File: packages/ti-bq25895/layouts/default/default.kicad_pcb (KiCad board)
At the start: 2 copper layers, 4 parts

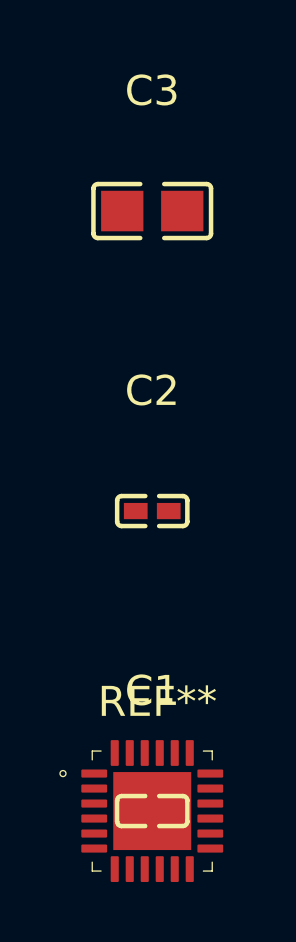
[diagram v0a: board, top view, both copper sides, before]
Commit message: adding has_part_picked trait to all
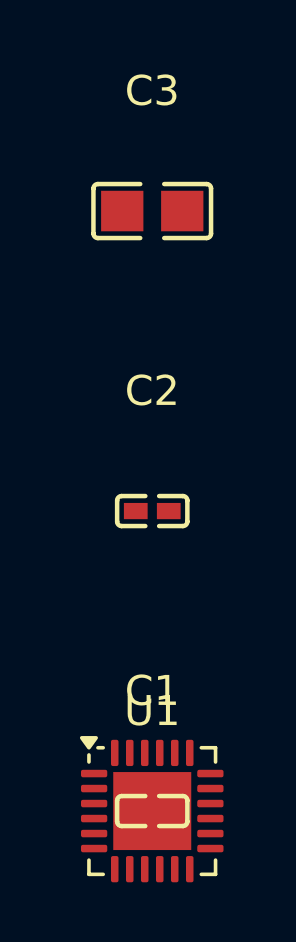
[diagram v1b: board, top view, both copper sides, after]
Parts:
- U1: footprint TI_BQ25895RTWR:QFN50P400X400X80-25N -> TI_BQ25895RTWR:WQFN-24-1EP_4x4mm_P0.5mm_EP2.6x2.6mm
